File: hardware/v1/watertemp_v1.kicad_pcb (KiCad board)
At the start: 2 copper layers, 4 parts, among them P1 CONN_01X08, P2 CONN_01X04, P3 CONN_01X07

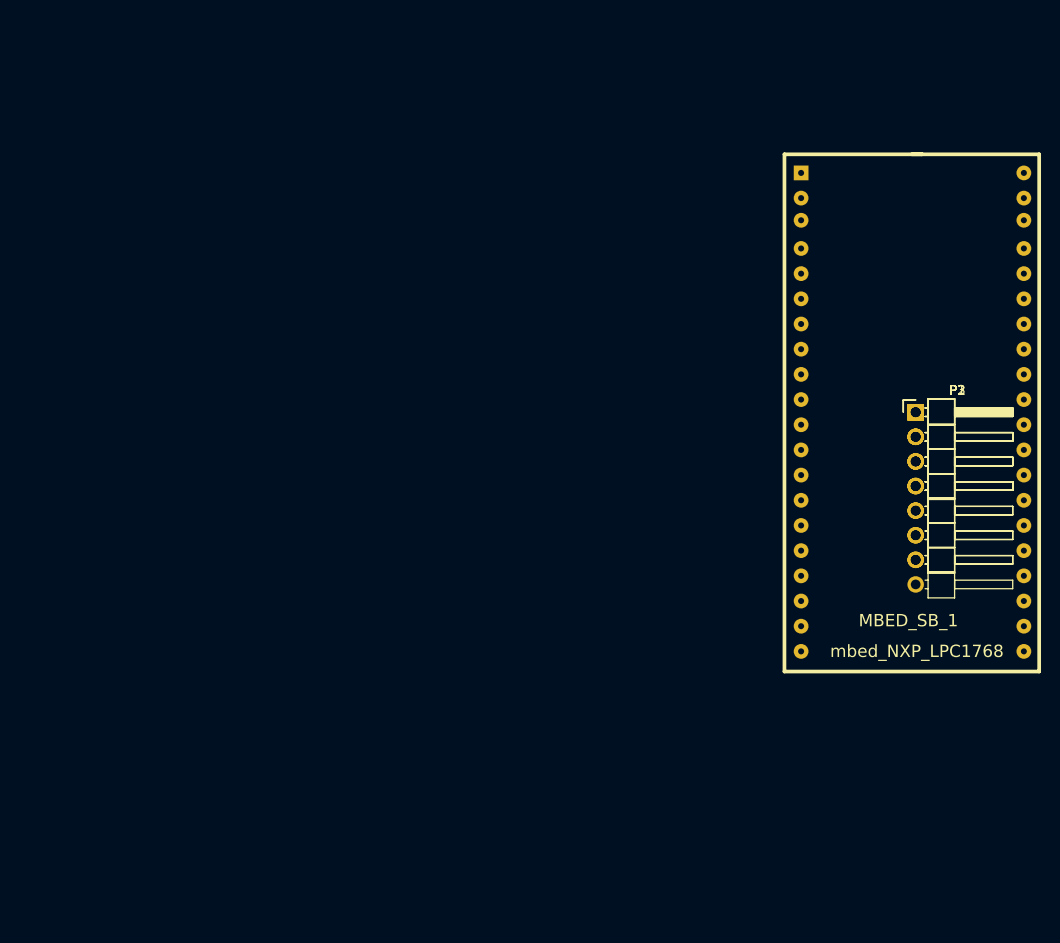
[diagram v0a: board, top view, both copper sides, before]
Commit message: PCB layouting
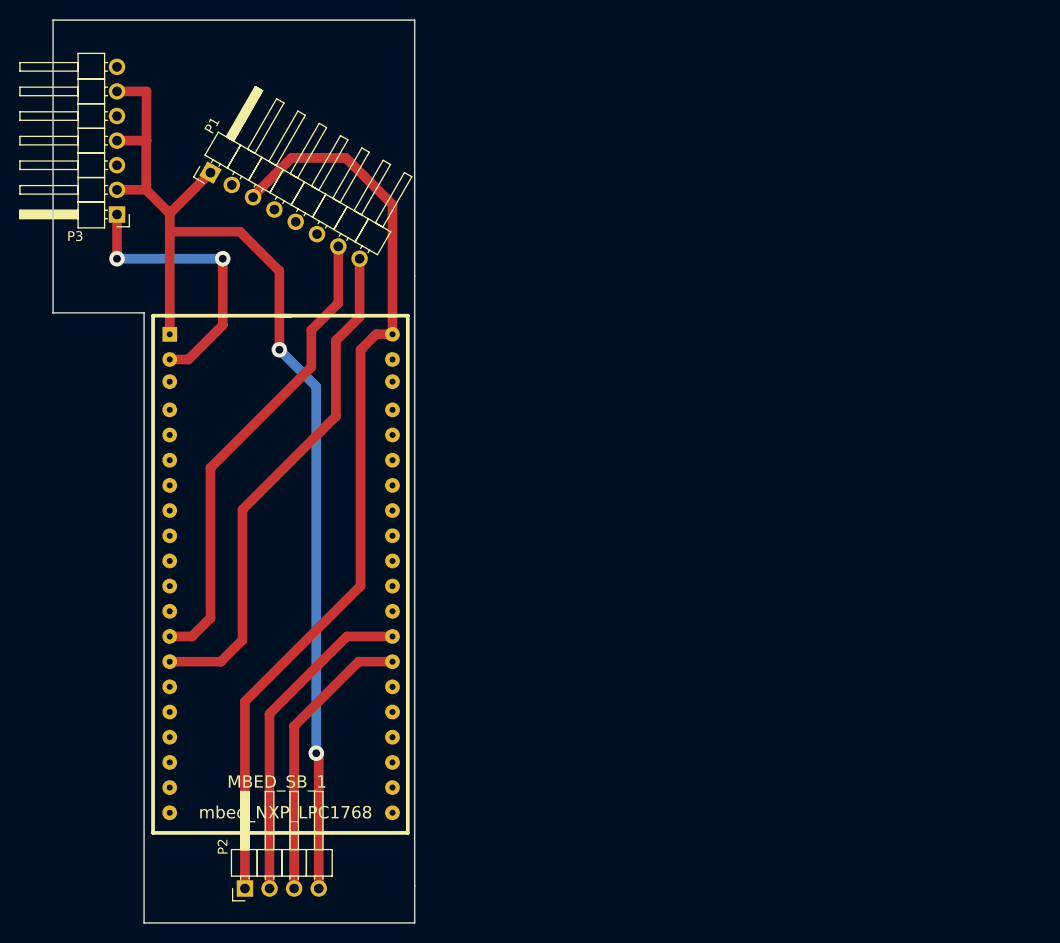
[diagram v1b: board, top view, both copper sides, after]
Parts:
- P1: value CONN_01X08 -> Lora
- P2: value CONN_01X04 -> Sensor
- P3: value CONN_01X07 -> Charger
- moved P3 85.0 mm to (66.0, 84.6), turned to 180 degrees
- moved P2 84.9 mm to (79.2, 154.2), turned to 90 degrees
- moved P1 76.9 mm to (75.7, 80.3), turned to 60 degrees
- moved MBED_SB_1 67.3 mm to (83.3, 121.7)
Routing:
- net GND: track 0.00 -> 119.6 mm, vias 0 -> 2
- net +3V3: track 0.00 -> 96.0 mm
- net Tx: track 0.00 -> 52.8 mm
- net Rx: track 0.00 -> 49.3 mm
- net /SDA: track 0.00 -> 34.0 mm
- net /SCL: track 0.00 -> 29.7 mm
- net +5V: track 0.00 -> 29.3 mm, vias 0 -> 2
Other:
- board outline added: 37.3 x 93.2 mm
- net class Default: clearance 0.2 -> 0.8; trace_width 0.25 -> 1; via_dia 0.6 -> 1.6; via_drill 0.4 -> 0.8
- rule trace_clearance: 0.2 -> 0.8
